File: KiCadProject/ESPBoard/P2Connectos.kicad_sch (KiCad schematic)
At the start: 27 parts, among them J201 Conn_02x05, J202 Conn_01x02, J203 Conn_02x05, J204 JST_SM04B, J205 DNP, J206 JST_B5B_XH, J207 JST_SM04B

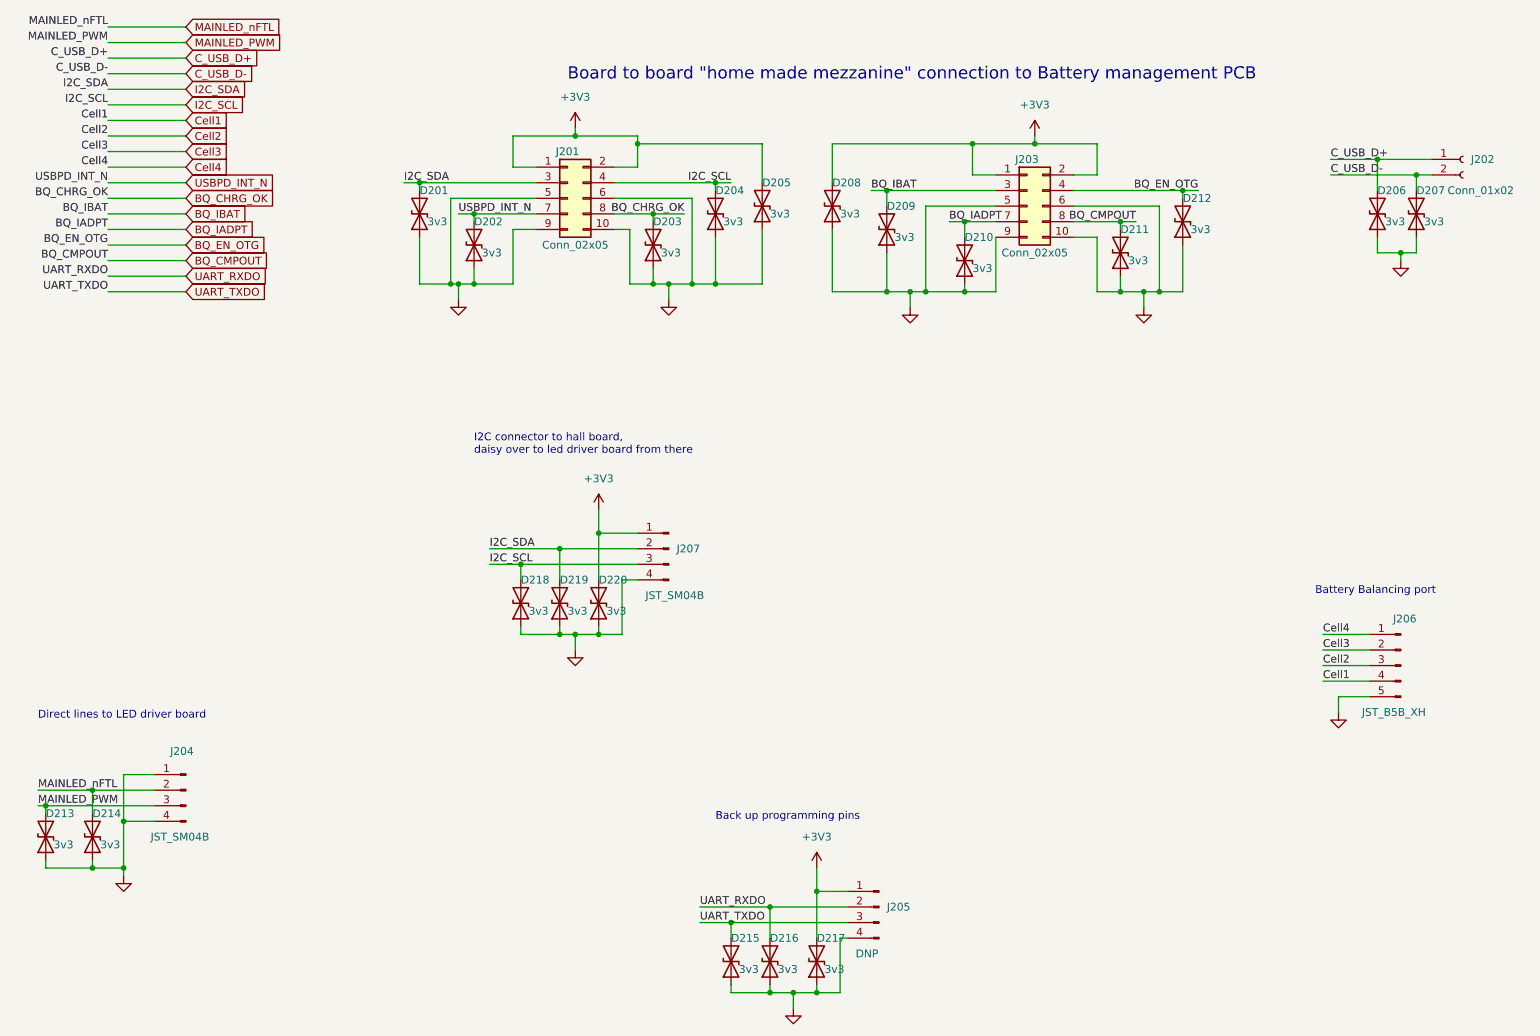
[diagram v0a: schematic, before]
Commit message: Tweaking
Signed-off-by: Eldalote.Electronics <Eldalote.Electronics@gmail.com>
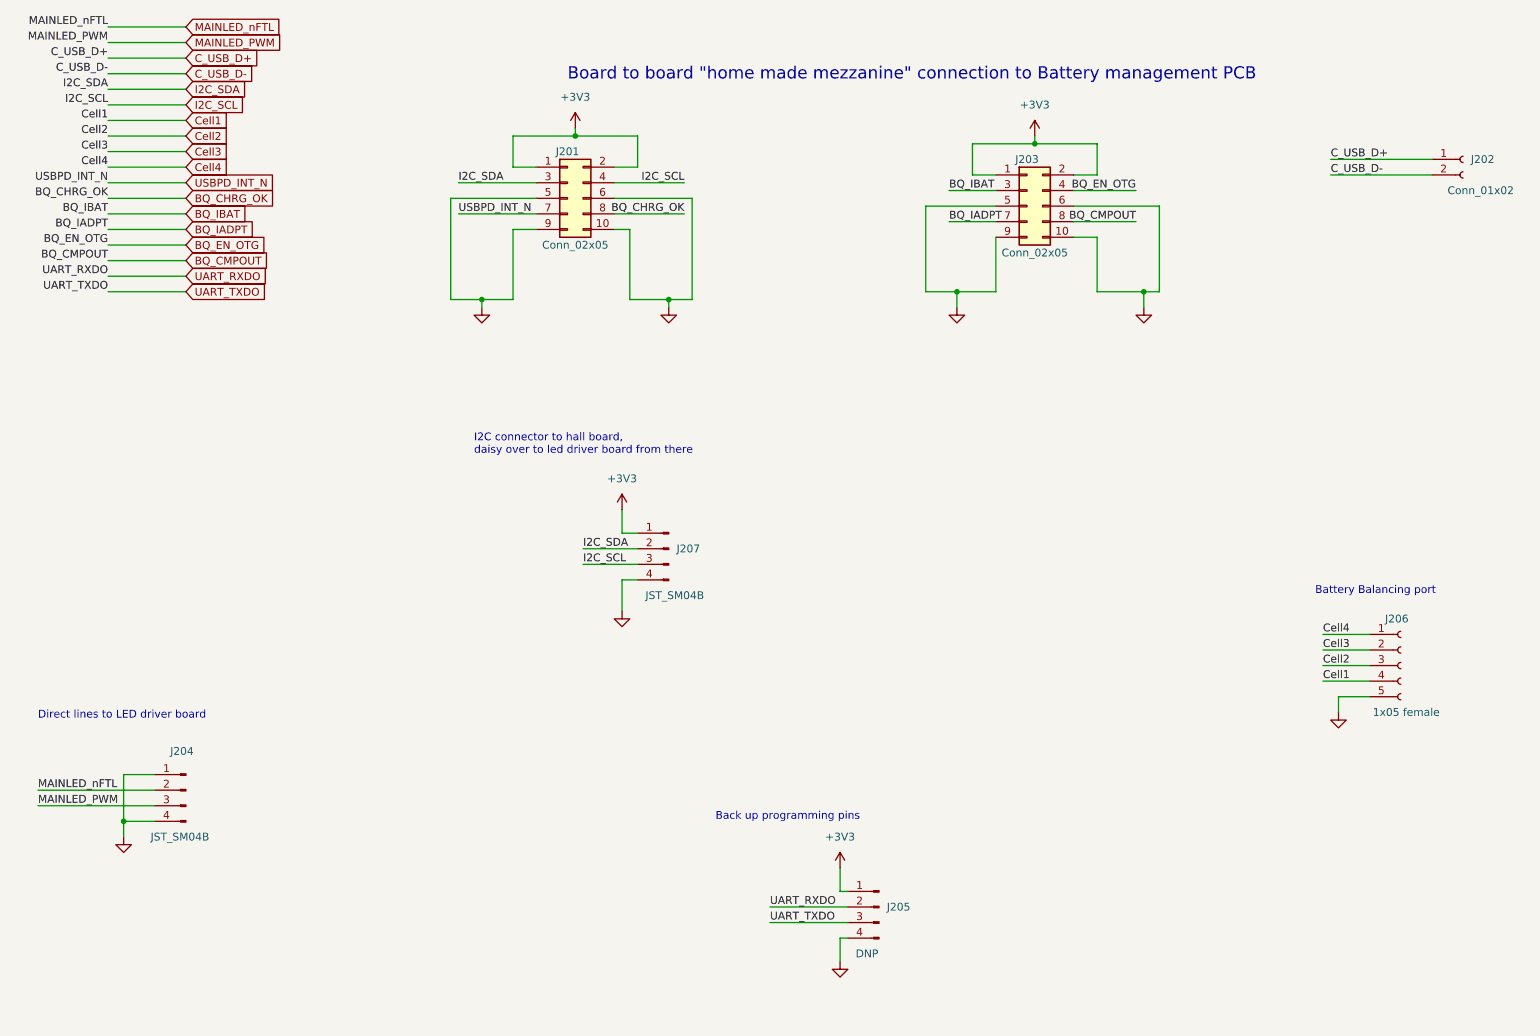
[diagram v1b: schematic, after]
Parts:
- removed D201, D202, D203, D204, D205, D206, D207, D208, D209, D210, D211, D212, D213, D214, D215, D216, D217, D218, D219, D220: 3v3, Diode_SMD:D_0402_1005Metric, symbol Device:D_TVS
- J205: footprint Connector_PinHeader_1.27mm:PinHeader_1x04_P1.27mm_Vertical -> Connector_PinHeader_1.27mm:PinHeader_2x02_P1.27mm_Vertical_SMD
- J206: value JST_B5B_XH -> 1x05 female; footprint Connector_JST:JST_XH_B5B-XH-A_1x05_P2.50mm_Vertical -> Connector_PinSocket_1.27mm:PinSocket_1x05_P1.27mm_Vertical_SMD_Pin1Left; symbol Connector:Conn_01x05_Male -> Connector:Conn_01x05_Female
